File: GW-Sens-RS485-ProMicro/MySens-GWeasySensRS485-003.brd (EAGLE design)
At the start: 33 x 40 mm, 19 parts, among them IC1 ATSHA204A, X7 1751264

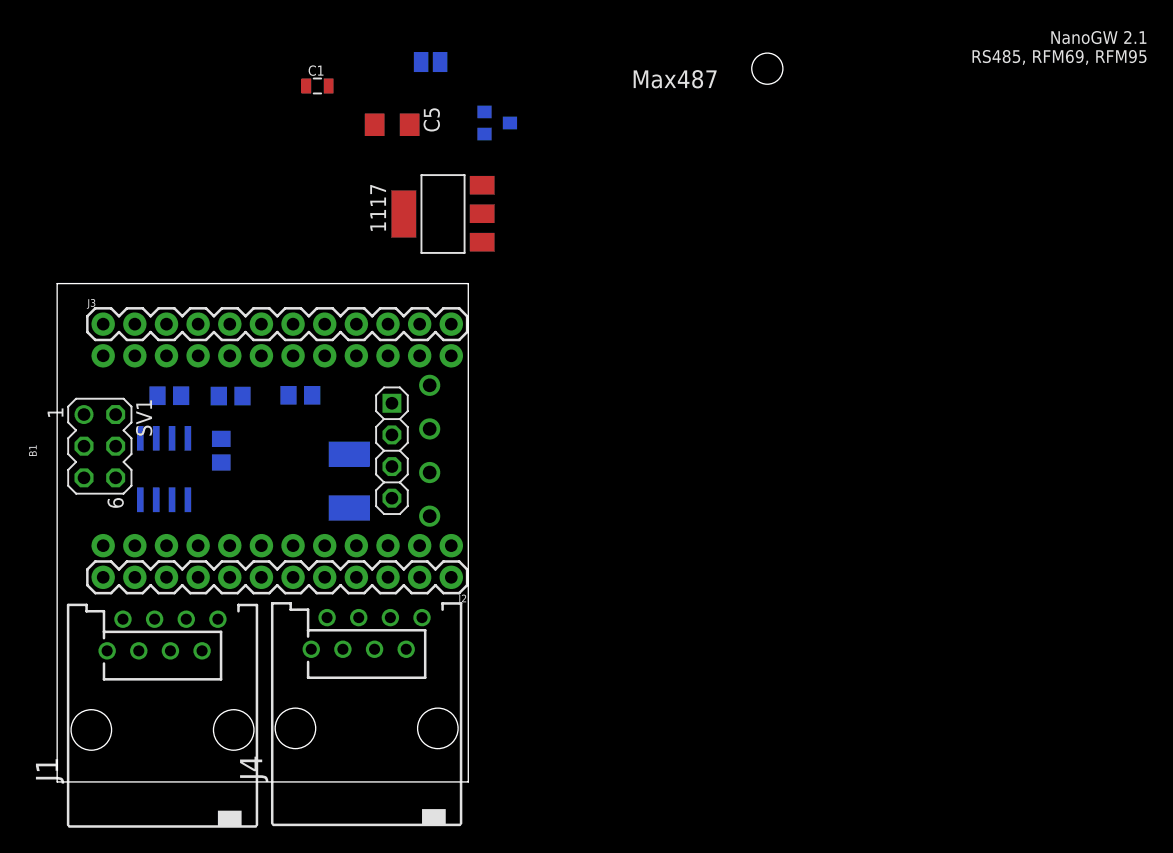
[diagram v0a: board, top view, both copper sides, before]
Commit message: RS485 Pro Mico ready for test
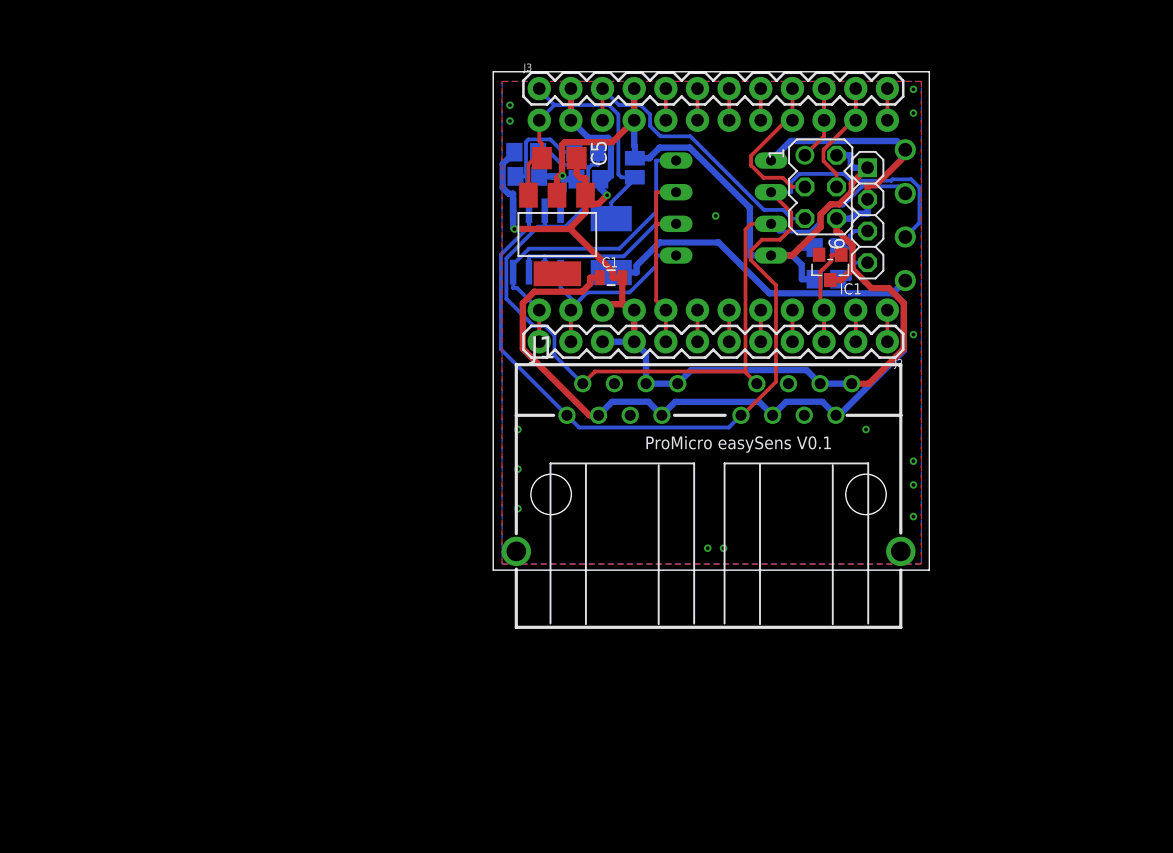
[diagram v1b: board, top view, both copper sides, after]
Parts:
- removed J4: (no value), con-amp:215878-2
- added MAX487: MAX481CPA, maxim-4:DIL08
- added R1, R2: 10K, rcl:R0805
- J1: device con-amp:215878-2 -> con-amp:557570-1
- moved SV1 61.5 mm to (26.3, 30.8)
- moved J1 47.8 mm to (17.3, 6.08)
- moved JP10 42.6 mm to (30.0, 28.5)
- moved X7 42.6 mm to (33.2, 28.5)
- moved B1 39.8 mm to (16.4, 28.5)
- moved J2 39.8 mm to (31.6, 18.3)
- moved J3 39.8 mm to (3.69, 38.6)
- moved C3 36.6 mm to (7.63, 31.4), turned to 0 degrees
- moved RS1 35.1 mm to (3.50, 26.4)
- moved R10 34.7 mm to (2.65, 33.5)
- moved R6 30.1 mm to (7.46, 33.6)
- moved R9 29.6 mm to (2.74, 31.6), turned to 0 degrees
- moved IC1 29.1 mm to (27.1, 24.3), flipped to the top, turned to 180 degrees
- moved F1 28.3 mm to (9.47, 26.1)
- moved C1 28.1 mm to (9.46, 23.5)
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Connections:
- removed net A4: JP10.4
- removed net A5: JP10.3
- removed net D7: IC1.1
- removed net RW: RAW.2
- new net D2: JP10.4, R1.2
- new net D3: JP10.3, R2.2
- net 7: now also IC1.1
- net A: now also J1.1-1, J1.2-1, MAX487.6; no longer J1.1, J4.1
- net B: now also J1.1-2, J1.2-2, MAX487.7; no longer J1.2, J4.2
- net GND: now also J1.1-6, J1.1-8, J1.2-6, J1.2-8, MAX487.5; no longer J1.6, J1.8, J4.6, J4.8
- net IN: now also J1.1-3, J1.1-7, J1.2-3, J1.2-7; no longer 1117.3, C5.1, J1.3, J1.7, J4.3, J4.7, RAW.1
- net IRQ: now also MAX487.2, MAX487.3
- net N$1: now also J1.2-4; no longer J4.4
- net N$10: now also J1.1-5; no longer J1.5
- net N$5: now also J1.2-5; no longer J4.5
- net N$9: now also J1.1-4; no longer J1.4
- net RAW: now also 1117.3, C5.1, RAW.2
- net RX: now also MAX487.1
- net TX: now also MAX487.4
- net VCC: now also MAX487.8, R1.1, R2.1, RAW.1
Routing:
- net GND: track 0.00 -> 112.0 mm, vias 0 -> 17
- net A: track 0.00 -> 86.0 mm
- net IN: track 0.00 -> 80.7 mm
- net B: track 0.00 -> 73.6 mm
- net VCC: track 0.00 -> 61.6 mm, vias 0 -> 1
- net IRQ: track 0.00 -> 31.0 mm
- net RAW: track 0.00 -> 26.3 mm
- net TX: track 0.00 -> 26.2 mm
- net RST: track 0.00 -> 23.6 mm
- net RX: track 0.00 -> 16.4 mm
- net SCK: track 0.00 -> 12.8 mm
- net MOSI: track 0.00 -> 9.51 mm
- net 7: track 0.00 -> 8.28 mm
- net MISO: track 0.00 -> 5.99 mm
- net D3: track 0.00 -> 3.46 mm
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- added copper zone on layer 1, net GND
- added copper zone on layer 16, net GND
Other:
- board size 33 x 40 mm -> 35 x 40 mm
- board text added: "A"
- board text added: "B"
- board text added: "D2"
- board text added: "D3"
- board text added: "Fuse"
- board text added: "GND"
- board text added: "ProMicro easySens V0.1"
- board text added: "VCC"
- board text added: "VIN"
- board text removed: "- B A +"
- board text removed: "Max487"
- board text removed: "NanoGW 2.1 RS485, RFM69, RFM95"
